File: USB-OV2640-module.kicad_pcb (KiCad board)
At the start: 2 copper layers, 43.5 x 32.7 mm, 116 parts, among them J1 USB_C_Receptacle_USB2.0_14P, J2 Conn_01x04_Pin, SW1 TS-1088-AR02016, SW2 TS-1088-AR02016, U1 USBLC6-2SC6, U2 XC6206-1.2V, U3 ESP32-S3, U4 XC6206-2.8V, U5 W25Q64JVSSIQ, Y1 XTM25040000JT00351005

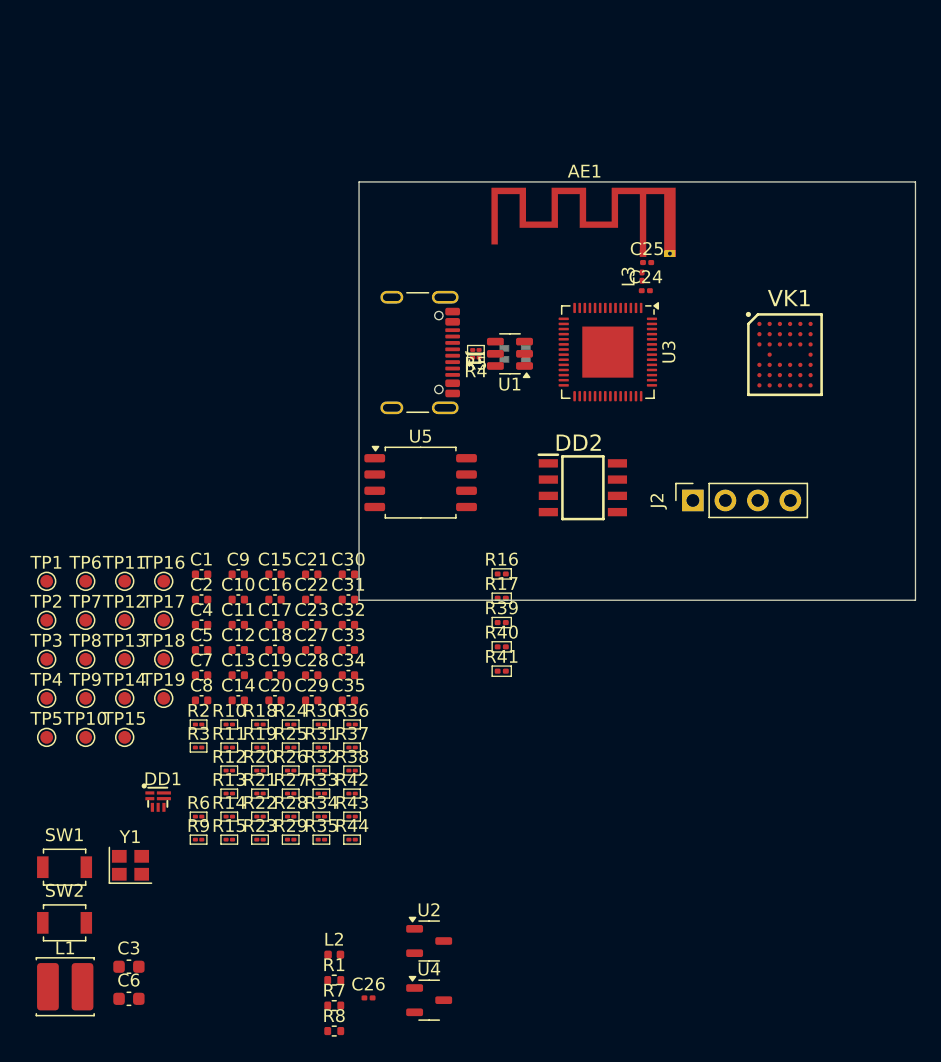
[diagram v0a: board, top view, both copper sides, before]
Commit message: Rev0 ready
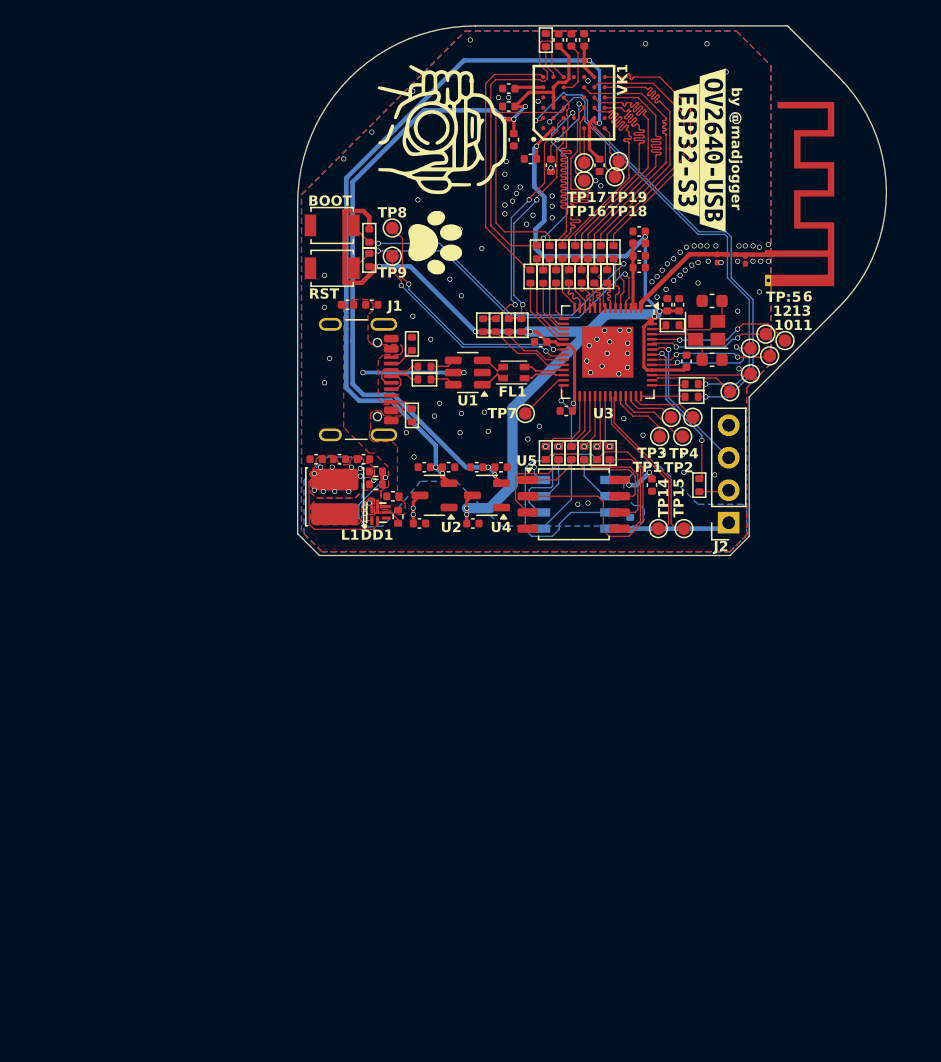
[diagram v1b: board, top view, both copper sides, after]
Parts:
- added G***: LOGO, LOGO, F.Cu at (101.7, 59.9)
- added G***: LOGO, LOGO, F.Cu at (101.4, 68.8)
- added G***: LOGO, LOGO, B.Cu at (112.7, 66.3)
- added kibuzzard-68B606AE: G***, kibuzzard-68B606AE, F.Cu at (121.1, 61.4)
- added kibuzzard-68B606C1: G***, kibuzzard-68B606C1, F.Cu at (123.2, 61.4)
- C26: footprint Capacitor_SMD:C_0201_0603Metric -> Capacitor_SMD:C_0402_1005Metric
- C29, DD2: moved to B.Cu
- FL1: moved to F.Cu
- R10, R11, R12, R13, R14, R15, R18, R19, R2, R20, R21, R22, R23, R24, R25, R26, R27, R28, R29, R3, R30, R31, R32, R33, R34, R35, R4, R5, R6, R9: footprint PCM_Resistor_SMD_AKL:R_01005_0402Metric -> PCM_Resistor_SMD_AKL:R_0402_1005Metric
- R16, R17, R39, R40, R41: footprint PCM_Resistor_SMD_AKL:R_0201_0603Metric -> PCM_Resistor_SMD_AKL:R_0402_1005Metric
- R36, R37, R38, R42, R43, R44: footprint PCM_Resistor_SMD_AKL:R_01005_0402Metric -> PCM_Resistor_SMD_AKL:R_0402_1005Metric; moved to B.Cu
- moved C3 69.2 mm to (123.1, 73.2)
- moved C6 67.6 mm to (123.1, 77.8), turned to 180 degrees
- moved C26 66.6 mm to (110.5, 62.6), turned to -90 degrees
- moved TP5 64.5 mm to (127.3, 75.8)
- moved Y1 61.5 mm to (122.7, 75.5)
- moved L2 60.5 mm to (117.4, 68.7), turned to 180 degrees
- moved BOOT 58.4 mm to (93.4, 67.3), turned to 180 degrees
- moved TP6 57.8 mm to (128.8, 76.3)
- moved TP10 57.2 mm to (124.5, 80.3)
- moved TP13 55.7 mm to (127.6, 77.5)
- moved TP4 55.1 mm to (121.6, 82.3)
- moved TP19 55.0 mm to (115.8, 62.3), turned to 180 degrees
- moved C28 53.6 mm to (112.1, 52.8), turned to 90 degrees
- moved R6 53.4 mm to (120.0, 75.1), turned to 180 degrees
- moved TP12 53.3 mm to (126.1, 76.9)
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- renumbered SW2 to BOOT, SW1 to RST
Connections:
- FL1 pad 1: USB_filter- -> USB_filter+
- FL1 pad 2: USB_mcu- -> USB_mcu+
- FL1 pad 3: USB_mcu+ -> USB_mcu-
- FL1 pad 4: USB_filter+ -> USB_filter-
- R18 pad 1: Y2 -> Y9
- R19 pad 1: Y3 -> Y8
- R20 pad 1: Y4 -> Y7
- R21 pad 1: Y5 -> Y6
- R22 pad 1: Y6 -> Y5
- R23 pad 1: Y7 -> Y4
- R24 pad 1: Y8 -> Y3
- R25 pad 1: Y9 -> Y2
- R4 pad 1: USB_res- -> USB_res+
- R4 pad 2: USB_con- -> USB_con+
- R40 pad 1: TWI_SCK -> SIO_D
- R41 pad 1: TWI_SDA -> SIO_C
- R5 pad 1: USB_res+ -> USB_res-
- R5 pad 2: USB_con+ -> USB_con-
- U1 pad 1: USB_filter- -> USB_filter+
- U1 pad 3: USB_filter+ -> USB_filter-
- U1 pad 4: USB_res+ -> USB_res-
- U1 pad 6: USB_res- -> USB_res+
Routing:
- net +3V3: track 0.00 -> 135.9 mm, vias 0 -> 24
- net +1V2: track 0.00 -> 65.8 mm, vias 0 -> 4
- net +2V8: track 0.00 -> 60.3 mm, vias 0 -> 5
- net EXPST_B: track 0.00 -> 38.8 mm, vias 0 -> 2
- net FREX: track 0.00 -> 36.1 mm, vias 0 -> 2
- net GPIO0: track 0.00 -> 29.6 mm, vias 0 -> 2
- net CHIP_PU: track 0.00 -> 28.2 mm, vias 0 -> 2
- net PCLK: track 0.00 -> 27.3 mm, vias 0 -> 2
- net RESETB: track 0.00 -> 27.1 mm
- net Y8: track 0.00 -> 22.8 mm
- net Y6: track 0.00 -> 22.7 mm
- net Y4: track 0.00 -> 22.7 mm
- net Y2: track 0.00 -> 22.7 mm
- net XVCLK: track 0.00 -> 22.6 mm
- net Y9: track 0.00 -> 21.6 mm
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- added copper zone on B.Cu, net +3V3
- added copper zone on F.Cu, net +3V3
- added copper zone on B.Cu, net Earth
- added copper zone on F.Cu, net Earth
- added copper zone on F.Cu, net Net-(DD1-LX)
- added copper zone on F.Cu, net VCC-5V
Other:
- board size 43.5 x 32.7 mm -> 46 x 41.4 mm
- board text added: "10"
- board text added: "11"
- board text added: "12"
- board text added: "13"
- board text added: "5"
- board text added: "6"
- board text added: "TP:"
- board text added: "by @madjogger"
